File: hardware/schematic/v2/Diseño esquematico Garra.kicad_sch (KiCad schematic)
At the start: 18 parts

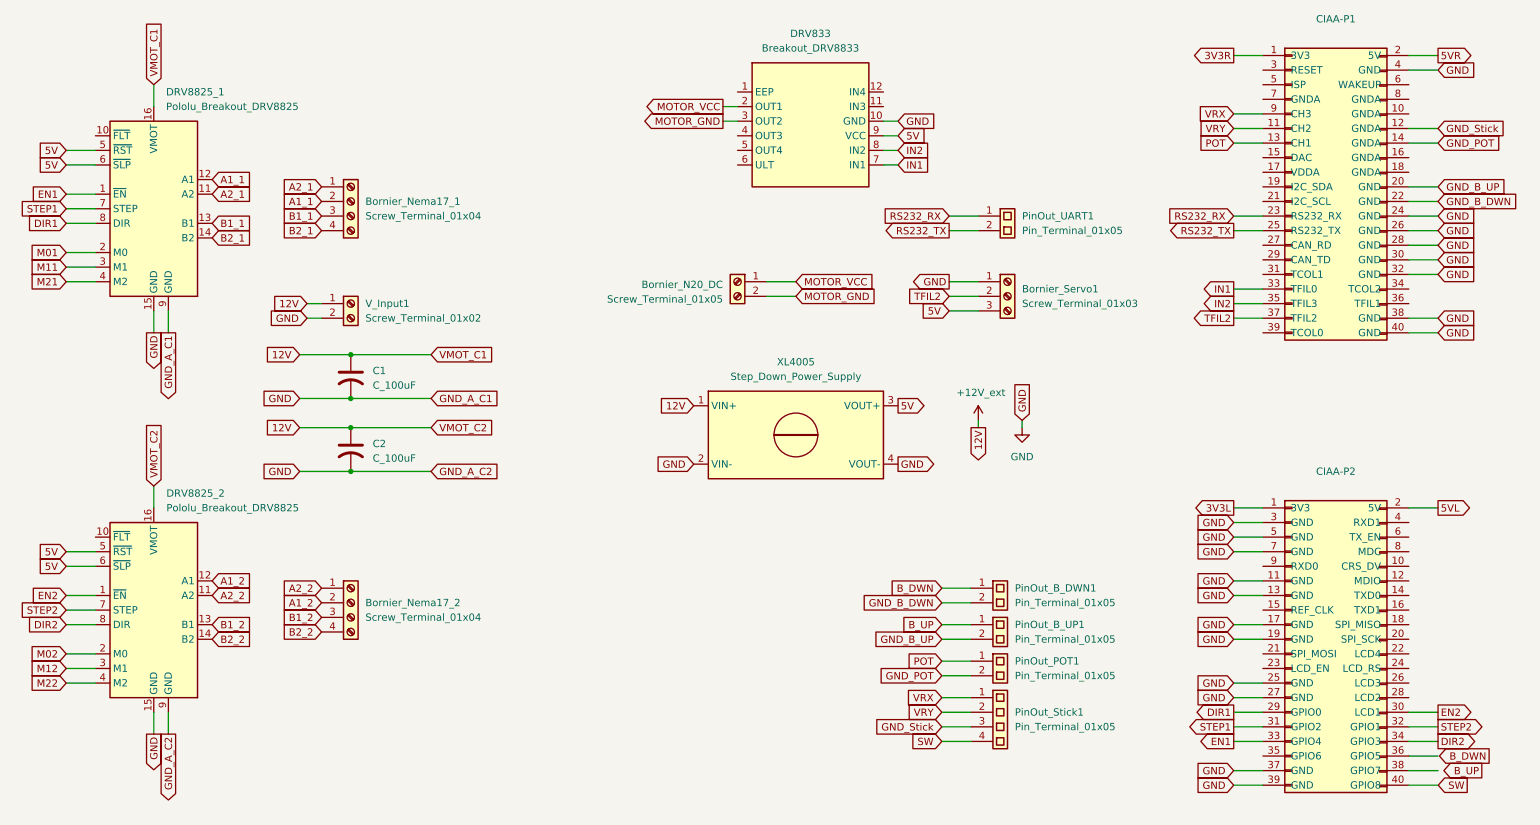
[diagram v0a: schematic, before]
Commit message: feat: PCB routing first stage completed
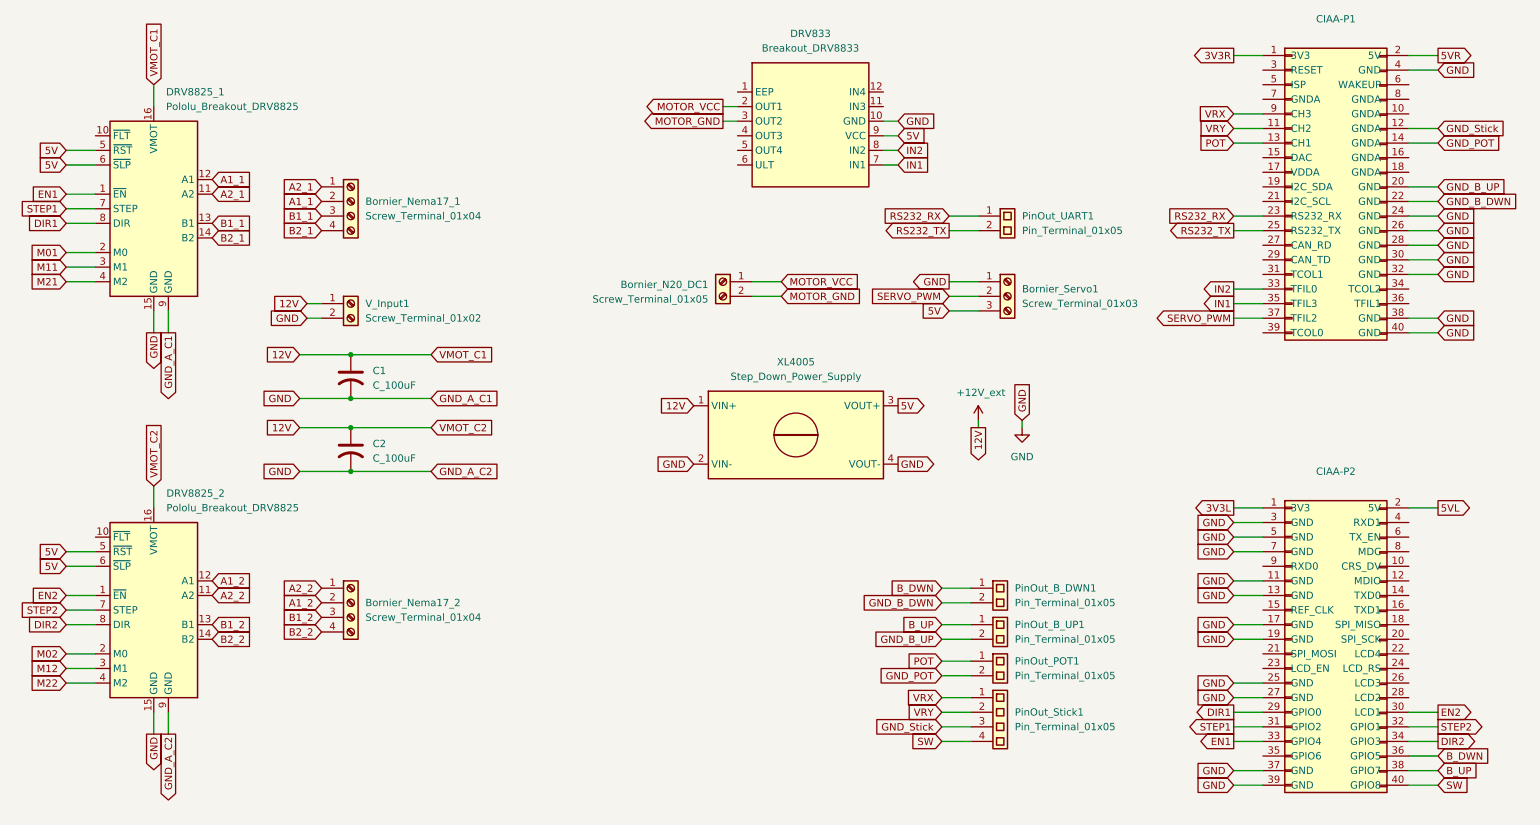
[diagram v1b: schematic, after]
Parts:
- renumbered Bornier_N20_DC to Bornier_N20_DC1
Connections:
- net B_DWN: now also CIAA-P2.36 (GPIO5)
- net B_UP: now also CIAA-P2.38 (GPIO7)
- net IN1: now also CIAA-P1.35 (TFIL3); no longer CIAA-P1.33 (TFIL0)
- net IN2: now also CIAA-P1.33 (TFIL0); no longer CIAA-P1.35 (TFIL3)
- net SW: now also CIAA-P2.40 (GPIO8)
- net TFIL2 renamed SERVO_PWM
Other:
- moved on the sheet: Bornier_N20_DC1
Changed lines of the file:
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@@
 	(wire
 		(pts
-			(xy 182.88 127) (xy 187.96 127)
+			(xy 264.16 146.05) (xy 269.24 146.05)
 		)
 		(stroke
@@
 	(wire
 		(pts
-			(xy 233.68 146.05) (xy 238.76 146.05)
+			(xy 182.88 127) (xy 187.96 127)
 		)
 		(stroke
@@
 	(wire
 		(pts
-			(xy 264.16 146.05) (xy 269.24 146.05)
+			(xy 233.68 146.05) (xy 238.76 146.05)
 		)
 		(stroke
@@
 	(wire
 		(pts
-			(xy 152.4 60.96) (xy 157.48 60.96)
+			(xy 149.86 60.96) (xy 154.94 60.96)
 		)
 		(stroke
@@
 	(wire
 		(pts
-			(xy 233.68 105.41) (xy 238.76 105.41)
+			(xy 264.16 143.51) (xy 269.24 143.51)
 		)
 		(stroke
@@
 	(wire
 		(pts
-			(xy 48.26 139.7) (xy 48.26 135.89)
+			(xy 233.68 105.41) (xy 238.76 105.41)
 		)
 		(stroke
@@
 	(wire
 		(pts
-			(xy 233.68 49.53) (xy 238.76 49.53)
+			(xy 48.26 139.7) (xy 48.26 135.89)
 		)
 		(stroke
@@
 	(wire
 		(pts
-			(xy 233.68 31.75) (xy 238.76 31.75)
+			(xy 233.68 49.53) (xy 238.76 49.53)
 		)
 		(stroke
@@
 	(wire
 		(pts
-			(xy 172.72 35.56) (xy 175.26 35.56)
+			(xy 233.68 31.75) (xy 238.76 31.75)
 		)
 		(stroke
@@
 	(wire
 		(pts
-			(xy 264.16 148.59) (xy 269.24 148.59)
+			(xy 172.72 35.56) (xy 175.26 35.56)
 		)
 		(stroke
@@
 	(wire
 		(pts
-			(xy 152.4 63.5) (xy 157.48 63.5)
+			(xy 149.86 63.5) (xy 154.94 63.5)
 		)
 		(stroke
@@
 	(wire
 		(pts
-			(xy 233.68 140.97) (xy 238.76 140.97)
+			(xy 264.16 148.59) (xy 269.24 148.59)
 		)
 		(stroke
@@
 	(wire
 		(pts
-			(xy 269.24 59.69) (xy 264.16 59.69)
+			(xy 233.68 140.97) (xy 238.76 140.97)
 		)
 		(stroke
@@
 	(wire
 		(pts
-			(xy 30.48 107.95) (xy 35.56 107.95)
+			(xy 269.24 59.69) (xy 264.16 59.69)
 		)
 		(stroke
@@
 	(wire
 		(pts
-			(xy 30.48 118.11) (xy 35.56 118.11)
+			(xy 30.48 107.95) (xy 35.56 107.95)
 		)
 		(stroke
@@
 	(wire
 		(pts
-			(xy 233.68 64.77) (xy 238.76 64.77)
+			(xy 30.48 118.11) (xy 35.56 118.11)
 		)
 		(stroke
@@
 	(wire
 		(pts
-			(xy 30.48 110.49) (xy 35.56 110.49)
+			(xy 233.68 64.77) (xy 238.76 64.77)
 		)
 		(stroke
@@
 	(wire
 		(pts
-			(xy 233.68 115.57) (xy 238.76 115.57)
+			(xy 30.48 110.49) (xy 35.56 110.49)
 		)
 		(stroke
@@
 	(wire
 		(pts
-			(xy 264.16 143.51) (xy 269.24 143.51)
+			(xy 233.68 115.57) (xy 238.76 115.57)
 		)
 		(stroke
@@
 		)
 	)
-	(global_label "B_UP"
+	(global_label "MOTOR_VCC"
 		(shape output)
-		(at 276.86 146.05 180)
+		(at 144.78 30.48 180)
 		(effects
 			(font
@@
 		)
 		(property "Intersheetrefs" "${INTERSHEET_REFS}"
-			(at 276.86 146.05 0)
+			(at 144.78 30.48 0)
 			(effects
 				(font
@@
 		)
 	)
-	(global_label "MOTOR_VCC"
-		(shape output)
-		(at 144.78 30.48 180)
+	(global_label "GND"
+		(shape input)
+		(at 269.24 67.31 0)
 		(effects
 			(font
 				(size 1.27 1.27)
 			)
-			(justify right)
+			(justify left)
 		)
 		(property "Intersheetrefs" "${INTERSHEET_REFS}"
-			(at 144.78 30.48 0)
+			(at 269.24 67.31 0)
 			(effects
 				(font
@@
 		)
 	)
-	(global_label "GND"
+	(global_label "GND_B_UP"
 		(shape input)
-		(at 269.24 67.31 0)
+		(at 182.88 123.19 180)
 		(effects
 			(font
 				(size 1.27 1.27)
 			)
-			(justify left)
+			(justify right)
 		)
 		(property "Intersheetrefs" "${INTERSHEET_REFS}"
-			(at 269.24 67.31 0)
+			(at 182.88 123.19 0)
 			(effects
 				(font
@@
 		)
 	)
-	(global_label "GND_B_UP"
+	(global_label "SW"
 		(shape input)
-		(at 182.88 123.19 180)
+		(at 269.24 148.59 0)
 		(effects
 			(font
 				(size 1.27 1.27)
 			)
-			(justify right)
+			(justify left)
 		)
 		(property "Intersheetrefs" "${INTERSHEET_REFS}"
-			(at 182.88 123.19 0)
+			(at 269.24 148.59 0)
 			(effects
 				(font
 					(size 1.27 1.27)
 				)
+				(justify left)
 				(hide yes)
 			)
@@
 		)
 	)
-	(global_label "B_DWN"
-		(shape output)
-		(at 278.13 143.51 180)
-		(effects
-			(font
-				(size 1.27 1.27)
-			)
-			(justify right)
-		)
-		(property "Intersheetrefs" "${INTERSHEET_REFS}"
-			(at 278.13 143.51 0)
-			(effects
-				(font
-					(size 1.27 1.27)
-				)
-				(hide yes)
-			)
-		)
-	)
 	(global_label "GND"
 		(shape input)
@@
 	(global_label "MOTOR_GND"
 		(shape input)
-		(at 157.48 63.5 0)
+		(at 154.94 63.5 0)
 		(effects
 			(font
@@
 		)
 		(property "Intersheetrefs" "${INTERSHEET_REFS}"
-			(at 157.48 63.5 0)
+			(at 154.94 63.5 0)
 			(effects
 				(font
@@
 		)
 	)
-	(global_label "TFIL2"
+	(global_label "SERVO_PWM"
 		(shape output)
 		(at 233.68 67.31 180)
@@
 		)
 	)
-	(global_label "SW"
-		(shape output)
-		(at 274.32 148.59 180)
-		(effects
-			(font
-				(size 1.27 1.27)
-			)
-			(justify right)
-		)
-		(property "Intersheetrefs" "${INTERSHEET_REFS}"
-			(at 274.32 148.59 0)
-			(effects
-				(font
-					(size 1.27 1.27)
-				)
-				(hide yes)
-			)
-		)
-	)
 	(global_label "M02"
 		(shape input)
@@
 		)
 	)
-	(global_label "TFIL2"
+	(global_label "B_DWN"
+		(shape input)
+		(at 269.24 143.51 0)
+		(effects
+			(font
+				(size 1.27 1.27)
+			)
+			(justify left)
+		)
+		(property "Intersheetrefs" "${INTERSHEET_REFS}"
+			(at 269.24 143.51 0)
+			(effects
+				(font
+					(size 1.27 1.27)
+				)
+				(justify left)
+				(hide yes)
+			)
+		)
+	)
+	(global_label "SERVO_PWM"
 		(shape input)
 		(at 184.15 63.5 180)
@@
 		)
 	)
-	(global_label "IN2"
+	(global_label "IN1"
 		(shape output)
 		(at 233.68 64.77 180)
@@
 	(global_label "MOTOR_VCC"
 		(shape input)
-		(at 157.48 60.96 0)
+		(at 154.94 60.96 0)
 		(effects
 			(font
@@
 		)
 		(property "Intersheetrefs" "${INTERSHEET_REFS}"
-			(at 157.48 60.96 0)
+			(at 154.94 60.96 0)
 			(effects
 				(font
@@
 		)
 	)
+	(global_label "B_UP"
+		(shape input)
+		(at 269.24 146.05 0)
+		(effects
+			(font
+				(size 1.27 1.27)
+			)
+			(justify left)
+		)
+		(property "Intersheetrefs" "${INTERSHEET_REFS}"
+			(at 269.24 146.05 0)
+			(effects
+				(font
+					(size 1.27 1.27)
+				)
+				(justify left)
+				(hide yes)
+			)
+		)
+	)
 	(global_label "A2_2"
 		(shape input)
@@
 		)
 	)
-	(global_label "IN1"
+	(global_label "IN2"
 		(shape output)
 		(at 233.68 62.23 180)
@@
 	(symbol
 		(lib_id "Connector:Screw_Terminal_01x02")
-		(at 147.32 60.96 0)
+		(at 144.78 60.96 0)
 		(mirror y)
 		(unit 1)
@@
 		(on_board yes)
 		(dnp no)
-		(property "Reference" "Bornier_N20_DC"
-			(at 144.78 61.468 0)
+		(property "Reference" "Bornier_N20_DC1"
+			(at 142.24 61.468 0)
 			(effects
 				(font
@@
 		)
 		(property "Value" "Screw_Terminal_01x05"
-			(at 144.78 64.008 0)
+			(at 142.24 64.008 0)
 			(effects
 				(font
@@
 		)
 		(property "Footprint" "TerminalBlock_Phoenix:TerminalBlock_Phoenix_MKDS-1,5-2-5.08_1x02_P5.08mm_Horizontal"
-			(at 147.32 60.96 0)
+			(at 144.78 60.96 0)
 			(effects
 				(font
@@
 		)
 		(property "Datasheet" "~"
-			(at 147.32 60.96 0)
+			(at 144.78 60.96 0)
 			(effects
 				(font
@@
 		)
 		(property "Description" "Generic screw terminal, single row, 01x02, script generated (kicad-library-utils/schlib/autogen/connector/)"
-			(at 147.32 60.96 0)
+			(at 144.78 60.96 0)
 			(effects
 				(font
@@
 			(project "Diseño esquematico Garra"
 				(path "/a88248f6-7b70-4a9d-b538-4e8e42a3a066"
-					(reference "Bornier_N20_DC")
+					(reference "Bornier_N20_DC1")
 					(unit 1)
 				)
